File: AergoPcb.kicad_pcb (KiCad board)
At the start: 2 copper layers, 299.2 x 140.2 mm, 245 parts, among them J1 Conn_01x15, J2 Conn_01x15, J3 Conn_01x04, M1 Mosfet-DMN63D8L, SW1 SW_Push, U1 ATmega32U4-AU, U2 PRTR5V0U2X, Y1 16MHz

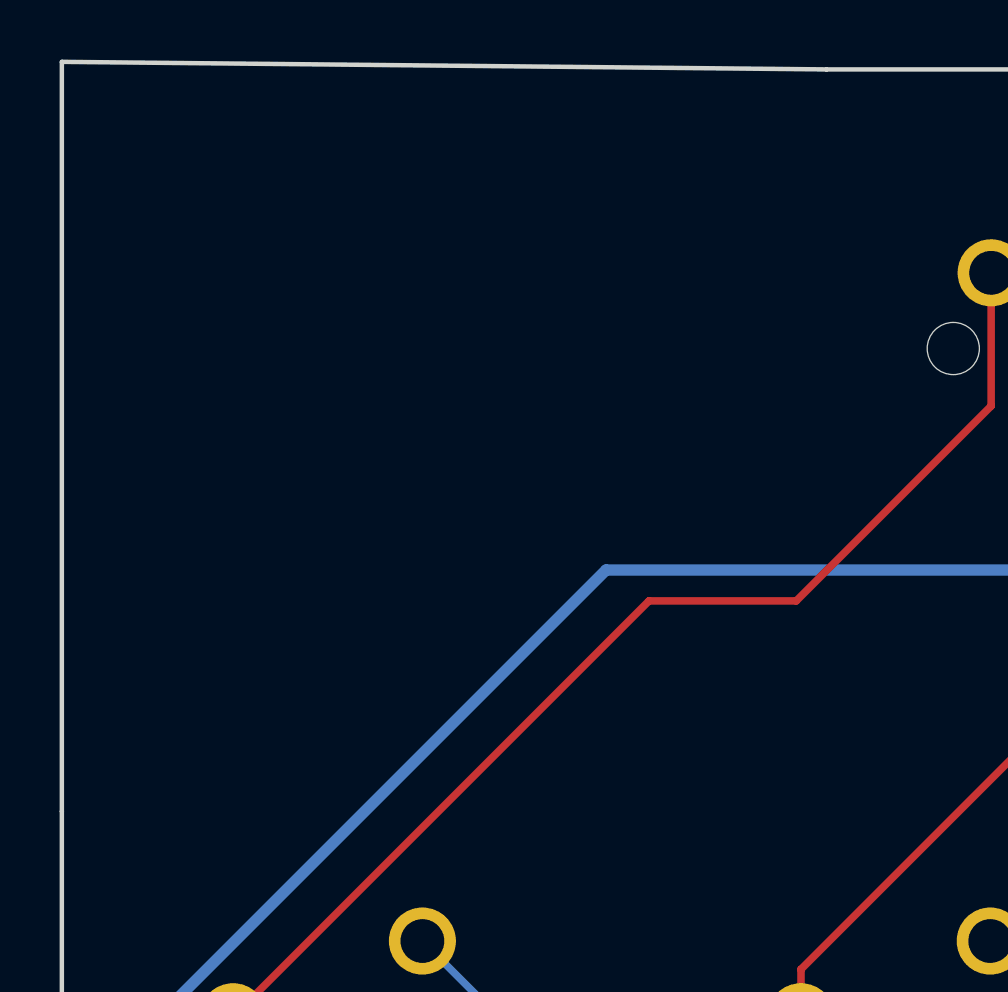
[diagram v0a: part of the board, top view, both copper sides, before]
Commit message: remade gerbers
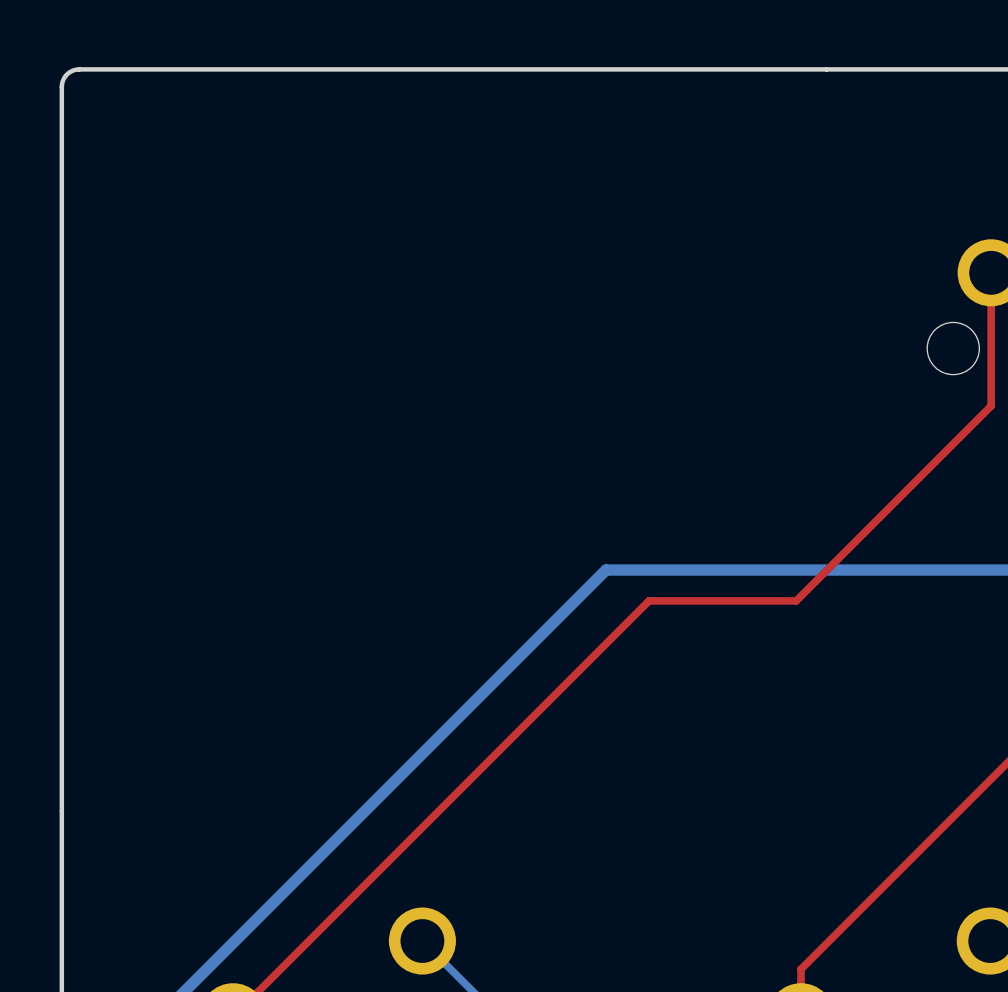
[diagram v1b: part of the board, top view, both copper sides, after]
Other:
- board size 299.2 x 140.2 mm -> 299.2 x 140 mm
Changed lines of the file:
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@@
   (general
     (thickness 1.6)
-    (drawings 61)
+    (drawings 60)
     (tracks 2344)
     (zones 0)
@@
       (net 2 GND))
   )
-  (dimension 120.2944 (width 0.3) (layer F.SilkS)
-    (gr_text "120.294 mm" (at 374.464 121.793 90) (layer F.SilkS)
-      (effects (font (size 1.5 1.5) (thickness 0.3)))
-    )
-    (feature1 (pts (xy 372.364 61.6458) (xy 372.950421 61.6458)))
-    (feature2 (pts (xy 372.364 181.9402) (xy 372.950421 181.9402)))
-    (crossbar (pts (xy 372.364 181.9402) (xy 372.364 61.6458)))
-    (arrow1a (pts (xy 372.364 61.6458) (xy 372.950421 62.772304)))
-    (arrow1b (pts (xy 372.364 61.6458) (xy 371.777579 62.772304)))
-    (arrow2a (pts (xy 372.364 181.9402) (xy 372.950421 180.813696)))
-    (arrow2b (pts (xy 372.364 181.9402) (xy 371.777579 180.813696)))
-  )
-  (dimension 299.365956 (width 0.3) (layer F.SilkS)
-    (gr_text "299.366 mm" (at 223.462347 64.329988 359.8152696) (layer F.SilkS)
-      (effects (font (size 1.5 1.5) (thickness 0.3)))
-    )
-    (feature1 (pts (xy 373.1514 62.6872) (xy 373.149427 63.299017)))
-    (feature2 (pts (xy 73.787 61.722) (xy 73.785027 62.333817)))
-    (crossbar (pts (xy 73.786918 61.747399) (xy 373.151318 62.712599)))
-    (arrow1a (pts (xy 373.151318 62.712599) (xy 372.022929 63.295385)))
-    (arrow1b (pts (xy 373.151318 62.712599) (xy 372.026711 62.122549)))
-    (arrow2a (pts (xy 73.786918 61.747399) (xy 74.911525 62.337449)))
-    (arrow2b (pts (xy 73.786918 61.747399) (xy 74.915307 61.164613)))
-  )
+  (gr_line (start 73.914 62.3062) (end 73.914 86.614) (layer Edge.Cuts) (width 0.15))
+  (gr_arc (start 74.4982 62.3062) (end 74.4982 61.722) (angle -90) (layer Edge.Cuts) (width 0.15))
+  (gr_line (start 99.568 61.722) (end 74.4982 61.722) (layer Edge.Cuts) (width 0.15))
   (gr_text "by AceRecon\n" (at 234.0356 172.6946) (layer F.SilkS)
     (effects (font (size 1.5 1.5) (thickness 0.3)))
@@
   (gr_line (start 118.618 61.722) (end 139.7 63.5) (layer Edge.Cuts) (width 0.15))
   (gr_line (start 99.568 61.722) (end 118.618 61.722) (layer Edge.Cuts) (width 0.15))
-  (gr_line (start 73.914 61.468) (end 99.568 61.722) (layer Edge.Cuts) (width 0.15))
-  (gr_line (start 73.914 86.614) (end 73.914 61.468) (layer Edge.Cuts) (width 0.15))
   (gr_line (start 73.914 180.848) (end 73.914 86.614) (layer Edge.Cuts) (width 0.15))
   (gr_arc (start 74.676 180.848) (end 73.914 180.848) (angle -90) (layer Edge.Cuts) (width 0.15))
